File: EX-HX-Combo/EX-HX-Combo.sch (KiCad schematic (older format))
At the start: 46 parts, among them CN1 DB9 Male, J1 IDE_CONNECTOR, J2 Bus_Tandy_Plus, J3 Bus_Tandy_Plus_Through, SW1 SW_DIP_x10, U1 BIOS FLASH, U2 74HCT245, U3 1.8432 MHz, U4 DS1315, U5 AS6C4008-55PCN, U6 16C550, U7 GD75232, U8 GAL16V8, U9 GAL16V8, Y1 32.768 kHz

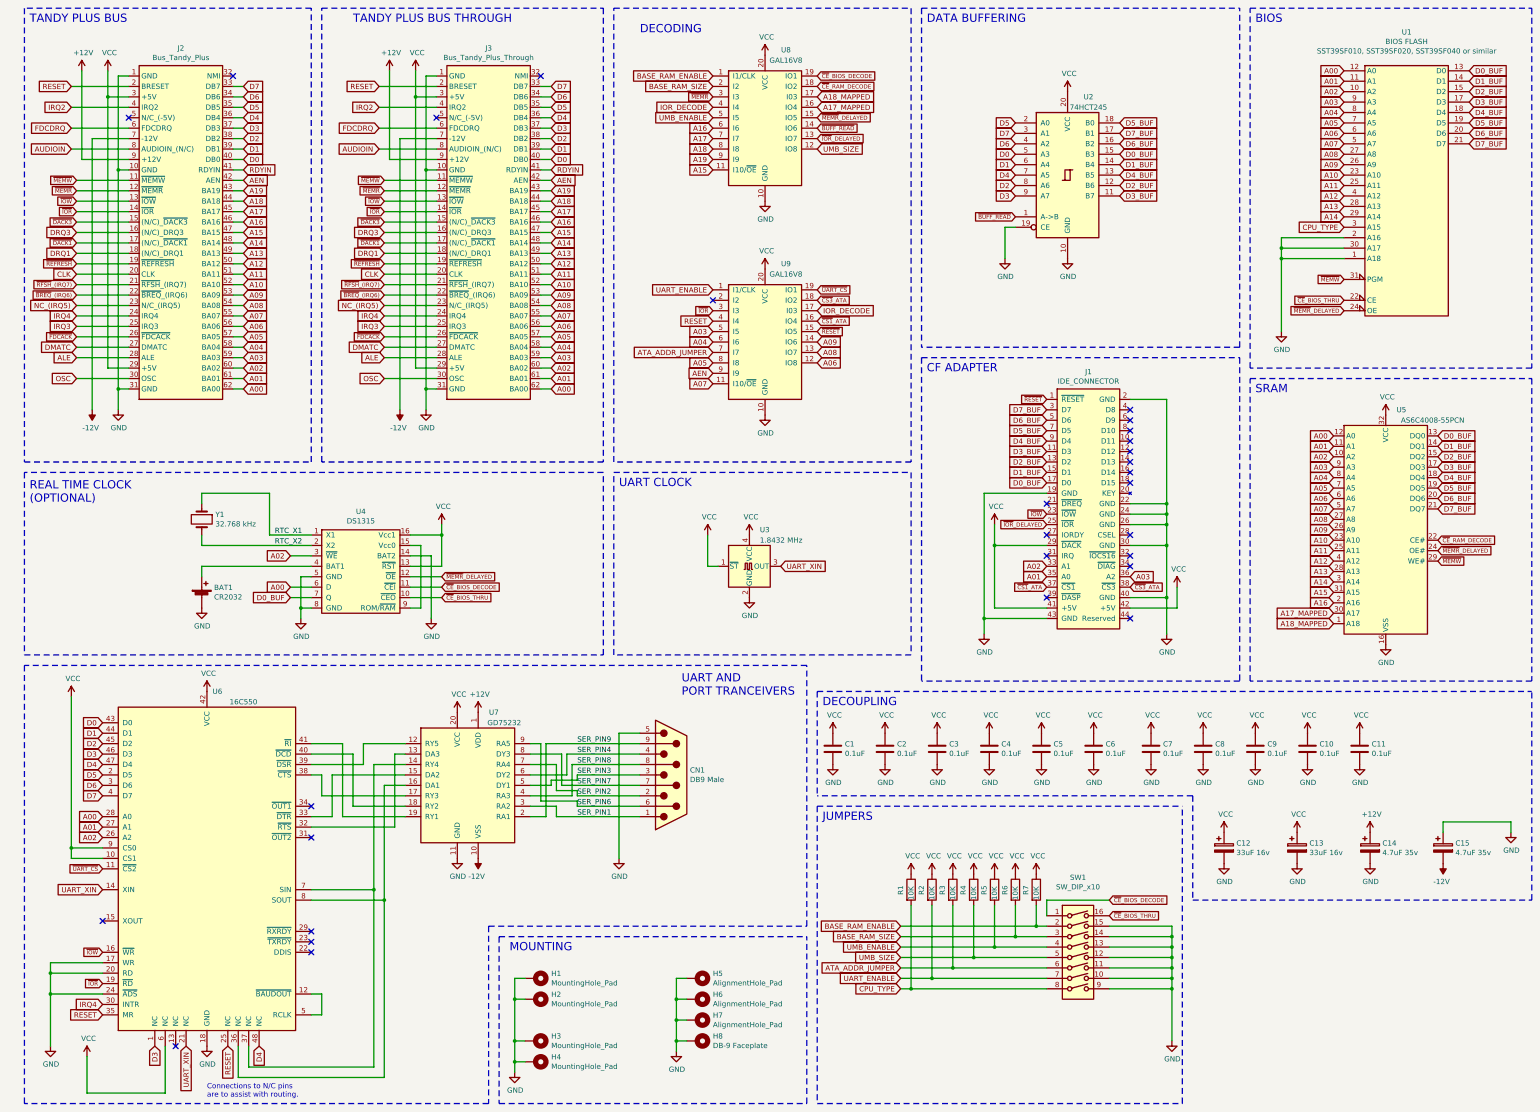
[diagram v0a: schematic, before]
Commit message: EX-HX-Combo: Various refinements.
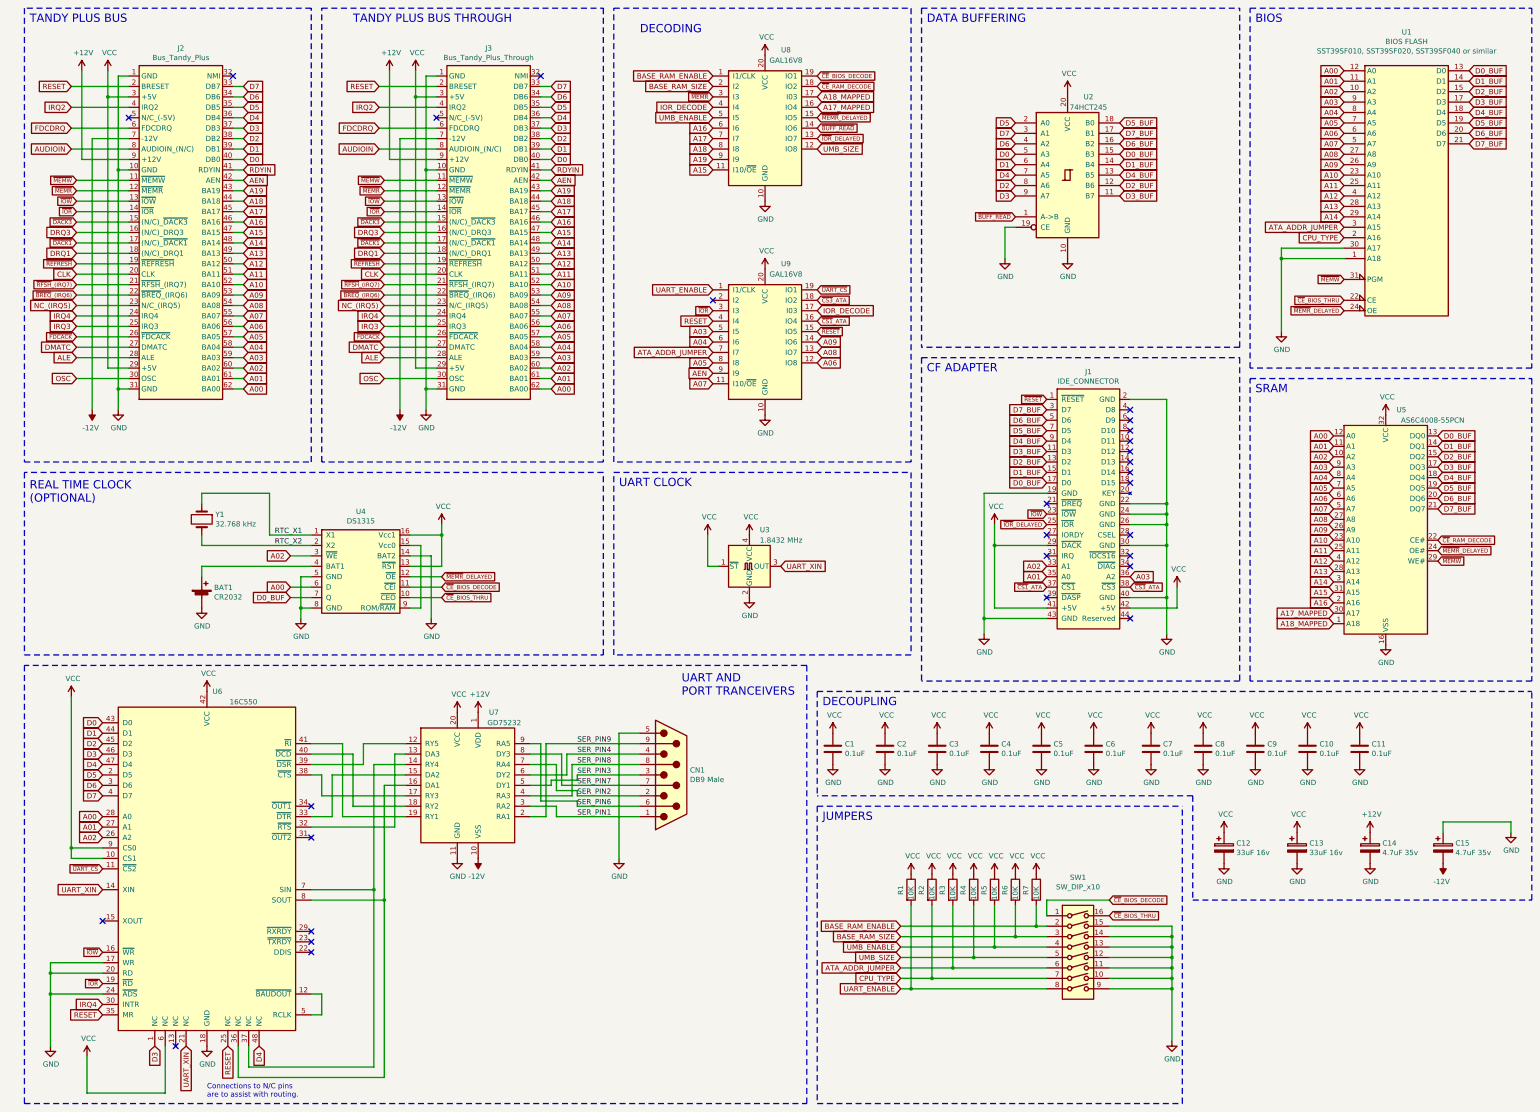
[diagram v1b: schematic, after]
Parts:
- removed H1, H2, H3, H4: MountingHole_Pad, MountingHole:MountingHole_3.5mm_Pad, symbol Mechanical:MountingHole_Pad
- removed H5, H6, H7: AlignmentHole_Pad, 00Custom:AlignmentHole, symbol Mechanical:MountingHole_Pad
- removed H8: DB-9 Faceplate, 00Custom:DB9_Face, symbol Mechanical:MountingHole_Pad
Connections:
- net ATA_ADDR_JUMPER: now also U1.3 (A15)
- net CPU_TYPE: now also R2.2, SW1.7, U1.2 (A16); no longer R1.2, SW1.8, U1.3 (A15)
- net GND: no longer U1.2 (A16)
- net UART_ENABLE: now also R1.2, SW1.8; no longer R2.2, SW1.7
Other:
- note removed: "MOUNTING"
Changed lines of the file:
@@
 Text GLabel 2700 2750 2    50   Input ~ 0
 A15
-Wire Wire Line
-	13250 2800 12650 2800
-Wire Wire Line
-	12650 2800 12650 2900
 Connection ~ 12650 3000
 Wire Wire Line
 	13250 2900 12650 2900
-Connection ~ 12650 2900
 Wire Wire Line
 	12650 2900 12650 3000
@@
 	1    0    0    -1
 $EndComp
-$Comp
-L Mechanical:MountingHole_Pad H1
-U 1 1 60D6AC46
-P 5500 9900
-F 0 "H1" V 5454 10050 50  0000 L CNN
-F 1 "MountingHole_Pad" V 5545 10050 50  0000 L CNN
-F 2 "MountingHole:MountingHole_3.5mm_Pad" H 5500 9900 50  0001 C CNN
-F 3 "~" H 5500 9900 50  0001 C CNN
-	1    5500 9900
-	0    1    1    0
-$EndComp
-$Comp
-L Mechanical:MountingHole_Pad H2
-U 1 1 60D6B05B
-P 5500 10100
-F 0 "H2" V 5454 10250 50  0000 L CNN
-F 1 "MountingHole_Pad" V 5545 10250 50  0000 L CNN
-F 2 "MountingHole:MountingHole_3.5mm_Pad" H 5500 10100 50  0001 C CNN
-F 3 "~" H 5500 10100 50  0001 C CNN
-	1    5500 10100
-	0    1    1    0
-$EndComp
-$Comp
-L Mechanical:MountingHole_Pad H3
-U 1 1 60D6B4F1
-P 5500 10500
-F 0 "H3" V 5454 10650 50  0000 L CNN
-F 1 "MountingHole_Pad" V 5545 10650 50  0000 L CNN
-F 2 "MountingHole:MountingHole_3.5mm_Pad" H 5500 10500 50  0001 C CNN
-F 3 "~" H 5500 10500 50  0001 C CNN
-	1    5500 10500
-	0    1    1    0
-$EndComp
-Wire Wire Line
-	5400 10500 5300 10500
-Connection ~ 5300 10500
-Wire Wire Line
-	5300 10500 5300 10700
-$Comp
-L Mechanical:MountingHole_Pad H4
-U 1 1 60D9AE58
-P 5500 10700
-F 0 "H4" V 5454 10850 50  0000 L CNN
-F 1 "MountingHole_Pad" V 5545 10850 50  0000 L CNN
-F 2 "MountingHole:MountingHole_3.5mm_Pad" H 5500 10700 50  0001 C CNN
-F 3 "~" H 5500 10700 50  0001 C CNN
-	1    5500 10700
-	0    1    1    0
-$EndComp
-Wire Wire Line
-	5400 10700 5300 10700
-Connection ~ 5300 10700
-Wire Wire Line
-	5300 10700 5300 10800
-$Comp
-L power:GND #PWR0148
-U 1 1 60DA739E
-P 5300 10800
-F 0 "#PWR0148" H 5300 10550 50  0001 C CNN
-F 1 "GND" H 5305 10627 50  0000 C CNN
-F 2 "" H 5300 10800 50  0001 C CNN
-F 3 "" H 5300 10800 50  0001 C CNN
-	1    5300 10800
-	1    0    0    -1
-$EndComp
-Wire Wire Line
-	5400 10100 5300 10100
-Connection ~ 5300 10100
-Wire Wire Line
-	5400 9900 5300 9900
-Wire Wire Line
-	5300 9900 5300 10100
 Text GLabel 5650 1350 2    50   Input ~ 0
 D7
@@
 Wire Wire Line
 	2600 2150 2700 2150
-Wire Wire Line
-	5300 10100 5300 10500
 Text GLabel 11000 9150 2    39   Input ~ 0
 ~CE~_BIOS_DECODE
@@
 Text GLabel 9000 9500 0    50   Input ~ 0
 BASE_RAM_SIZE
+Text GLabel 9000 9900 0    50   Input ~ 0
+CPU_TYPE
 Text GLabel 9000 10000 0    50   Input ~ 0
-CPU_TYPE
-Text GLabel 9000 9900 0    50   Input ~ 0
 UART_ENABLE
 Text GLabel 11100 2000 2    50   Input ~ 0
@@
 	1    0    0    -1
 $EndComp
-$Comp
-L Mechanical:MountingHole_Pad H5
-U 1 1 61187FCA
-P 7050 9900
-F 0 "H5" V 7004 10050 50  0000 L CNN
-F 1 "AlignmentHole_Pad" V 7095 10050 50  0000 L CNN
-F 2 "00Custom:AlignmentHole" H 7050 9900 50  0001 C CNN
-F 3 "~" H 7050 9900 50  0001 C CNN
-	1    7050 9900
-	0    1    1    0
-$EndComp
-$Comp
-L Mechanical:MountingHole_Pad H6
-U 1 1 611A4105
-P 7050 10100
-F 0 "H6" V 7004 10250 50  0000 L CNN
-F 1 "AlignmentHole_Pad" V 7095 10250 50  0000 L CNN
-F 2 "00Custom:AlignmentHole" H 7050 10100 50  0001 C CNN
-F 3 "~" H 7050 10100 50  0001 C CNN
-	1    7050 10100
-	0    1    1    0
-$EndComp
-$Comp
-L Mechanical:MountingHole_Pad H7
-U 1 1 611C6C9E
-P 7050 10300
-F 0 "H7" V 7004 10450 50  0000 L CNN
-F 1 "AlignmentHole_Pad" V 7095 10450 50  0000 L CNN
-F 2 "00Custom:AlignmentHole" H 7050 10300 50  0001 C CNN
-F 3 "~" H 7050 10300 50  0001 C CNN
-	1    7050 10300
-	0    1    1    0
-$EndComp
-Wire Wire Line
-	6950 9900 6850 9900
-Wire Wire Line
-	6850 9900 6850 10100
-$Comp
-L power:GND #PWR0179
-U 1 1 6120C5C6
-P 6850 10600
-F 0 "#PWR0179" H 6850 10350 50  0001 C CNN
-F 1 "GND" H 6855 10427 50  0000 C CNN
-F 2 "" H 6850 10600 50  0001 C CNN
-F 3 "" H 6850 10600 50  0001 C CNN
-	1    6850 10600
-	1    0    0    -1
-$EndComp
-Wire Wire Line
-	6950 10100 6850 10100
-Connection ~ 6850 10100
-Wire Wire Line
-	6850 10100 6850 10300
-Wire Wire Line
-	6950 10300 6850 10300
-Connection ~ 6850 10300
-$Comp
-L Mechanical:MountingHole_Pad H8
-U 1 1 611975A0
-P 7050 10500
-F 0 "H8" V 7004 10650 50  0000 L CNN
-F 1 "DB-9 Faceplate" V 7095 10650 50  0000 L CNN
-F 2 "00Custom:DB9_Face" H 7050 10500 50  0001 C CNN
-F 3 "~" H 7050 10500 50  0001 C CNN
-	1    7050 10500
-	0    1    1    0
-$EndComp
-Wire Wire Line
-	6850 10300 6850 10500
-Wire Wire Line
-	6950 10500 6850 10500
-Connection ~ 6850 10500
-Wire Wire Line
-	6850 10500 6850 10600
 Wire Wire Line
 	10400 9300 10400 9150
@@
 	1    0    0    -1
 $EndComp
-Text Notes 5250 9650 0    79   ~ 0
-MOUNTING
-Wire Notes Line
-	5150 9500 5150 11100
-Wire Notes Line
-	5150 9500 8100 9500
-Wire Notes Line
-	5050 9400 8100 9400
-Wire Notes Line
-	5050 9400 5050 11100
-Wire Notes Line
-	5050 11100 600  11100
-Wire Notes Line
-	5150 11100 8100 11100
-Wire Notes Line
-	8100 11100 8100 9500
-Wire Notes Line
-	8100 9400 8100 6900
+Wire Notes Line
+	8100 11100 8100 6900
 Wire Notes Line
 	11800 8150 11800 9150
@@
 Wire Wire Line
 	1600 3650 1100 3650
+Text GLabel 13250 2800 0    50   Input ~ 0
+CPU_TYPE
+Wire Notes Line
+	600  11100 8100 11100
 Text GLabel 13250 2700 0    50   Input ~ 0
-CPU_TYPE
+ATA_ADDR_JUMPER
 $EndSCHEMATC
